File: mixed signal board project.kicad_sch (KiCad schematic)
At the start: 0 parts

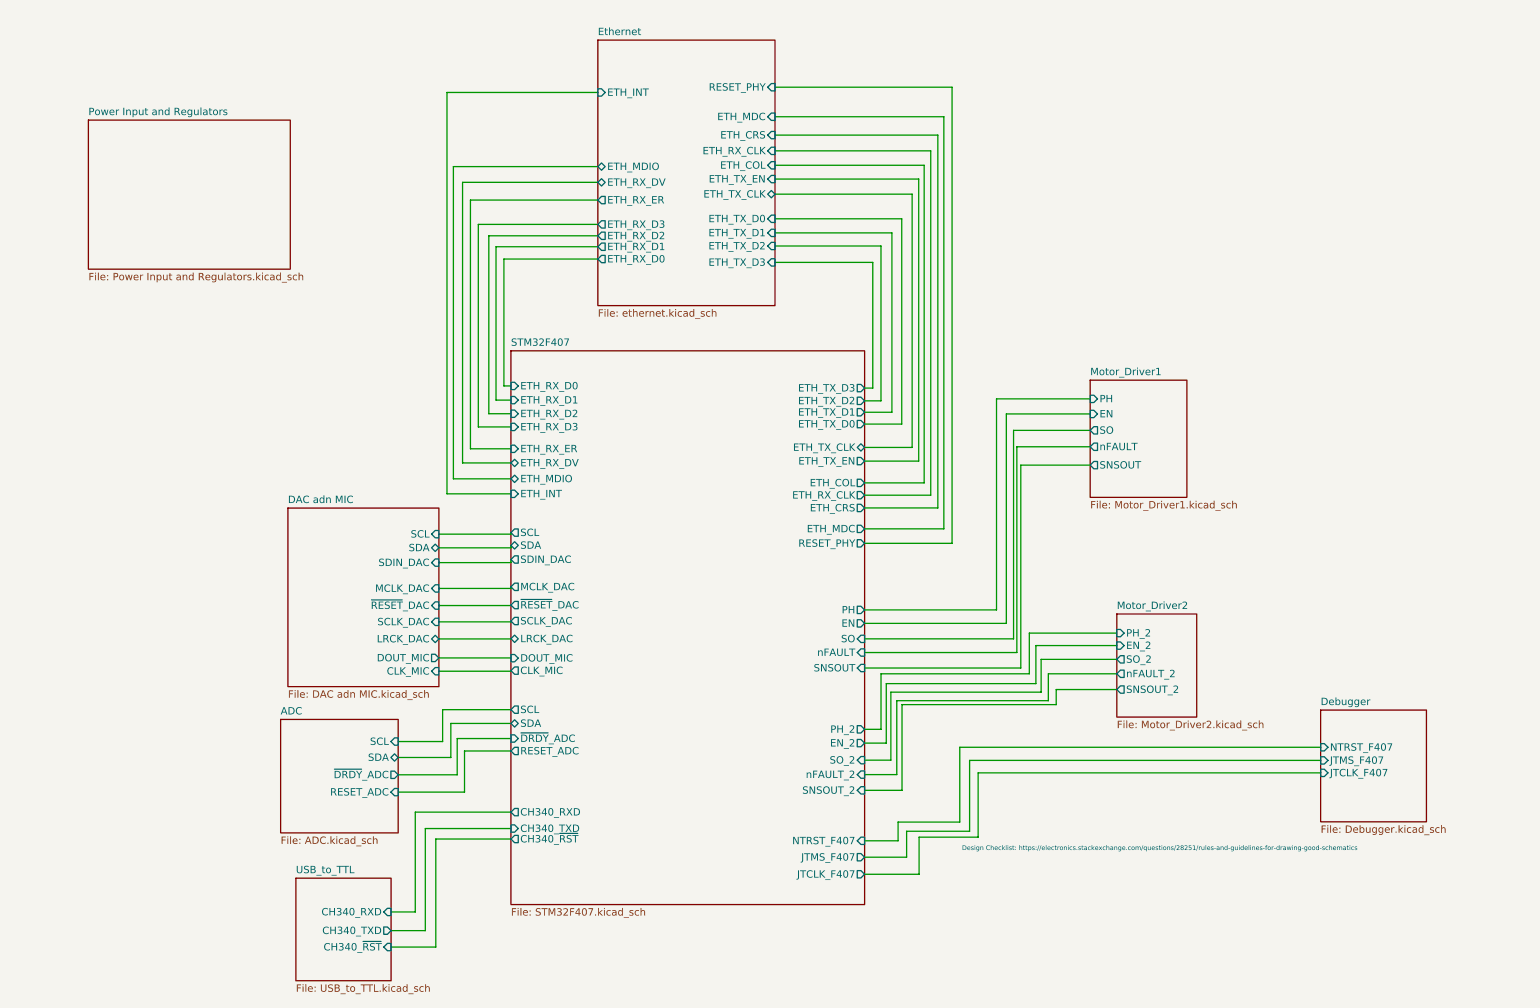
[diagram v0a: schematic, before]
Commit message: schematic pages are reviewed
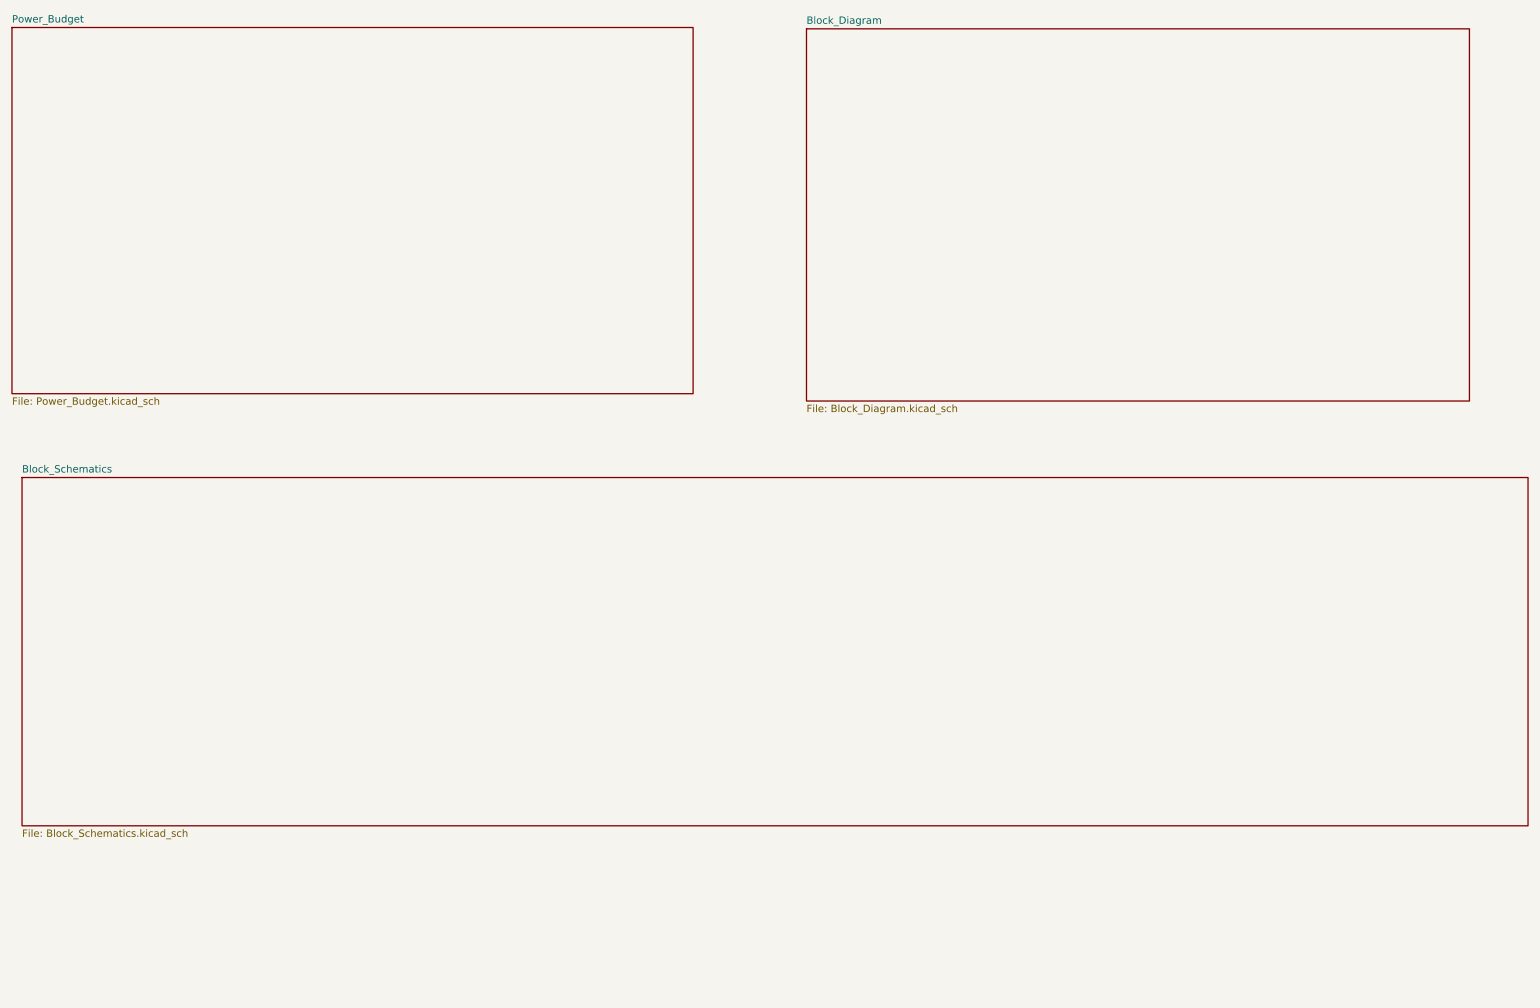
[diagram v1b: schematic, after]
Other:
- removed sheet ADC
- removed sheet DAC adn MIC
- removed sheet Debugger
- removed sheet Ethernet
- removed sheet Motor_Driver1
- removed sheet Motor_Driver2
- removed sheet Power Input and Regulators
- removed sheet STM32F407
- removed sheet USB_to_TTL
- added sheet Block_Diagram (Block_Diagram.kicad_sch)
- added sheet Block_Schematics (Block_Schematics.kicad_sch)
- added sheet Power_Budget (Power_Budget.kicad_sch)
- note removed: "Design Checklist: https://electronics.stackexchange.com/questions/28251/rules-and-guidelines-for-drawing-good-schematics"
